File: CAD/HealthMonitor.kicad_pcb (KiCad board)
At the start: 2 copper layers, 20 x 30 mm, 28 parts, among them J1 USB_C_Receptacle_USB2.0, U1 ADP5092ACPZ-1-R7, U2 LTC4079IDD-PBF

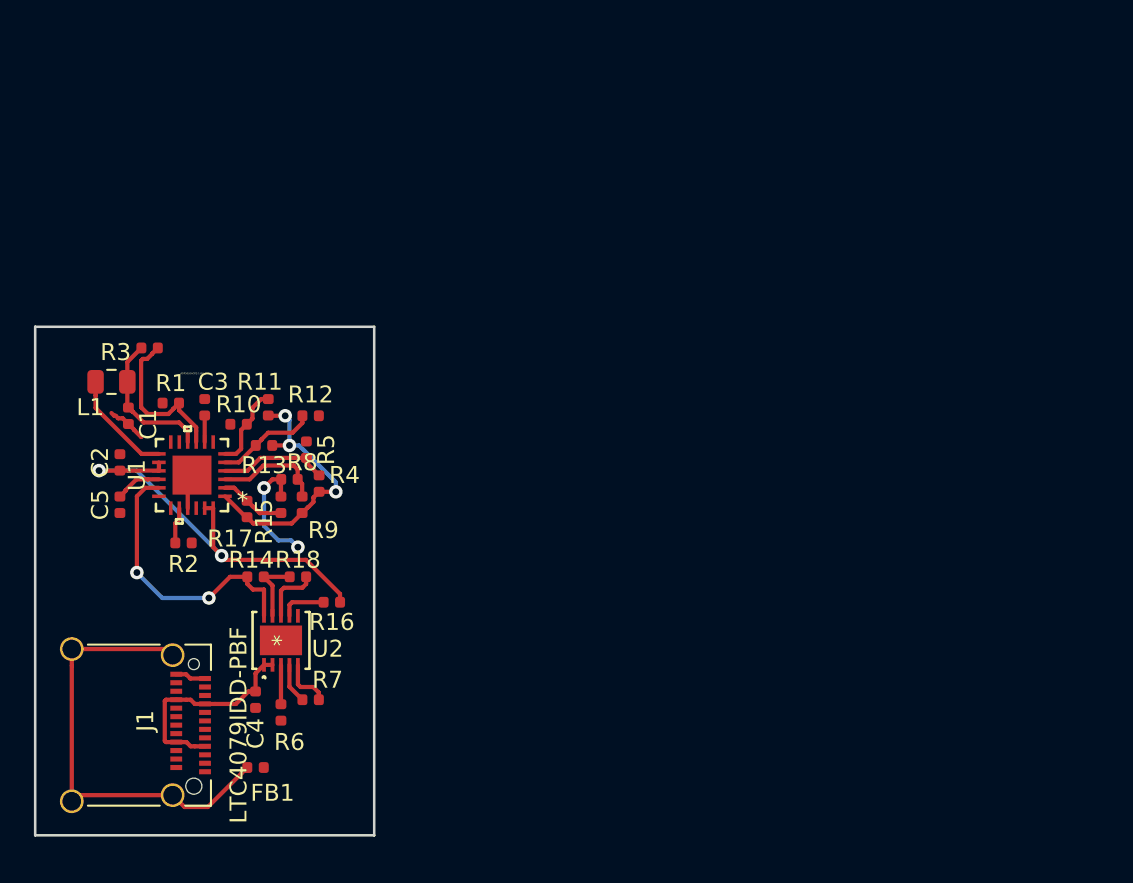
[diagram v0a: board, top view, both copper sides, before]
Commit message: Finished PCB Draft -- waiting for review
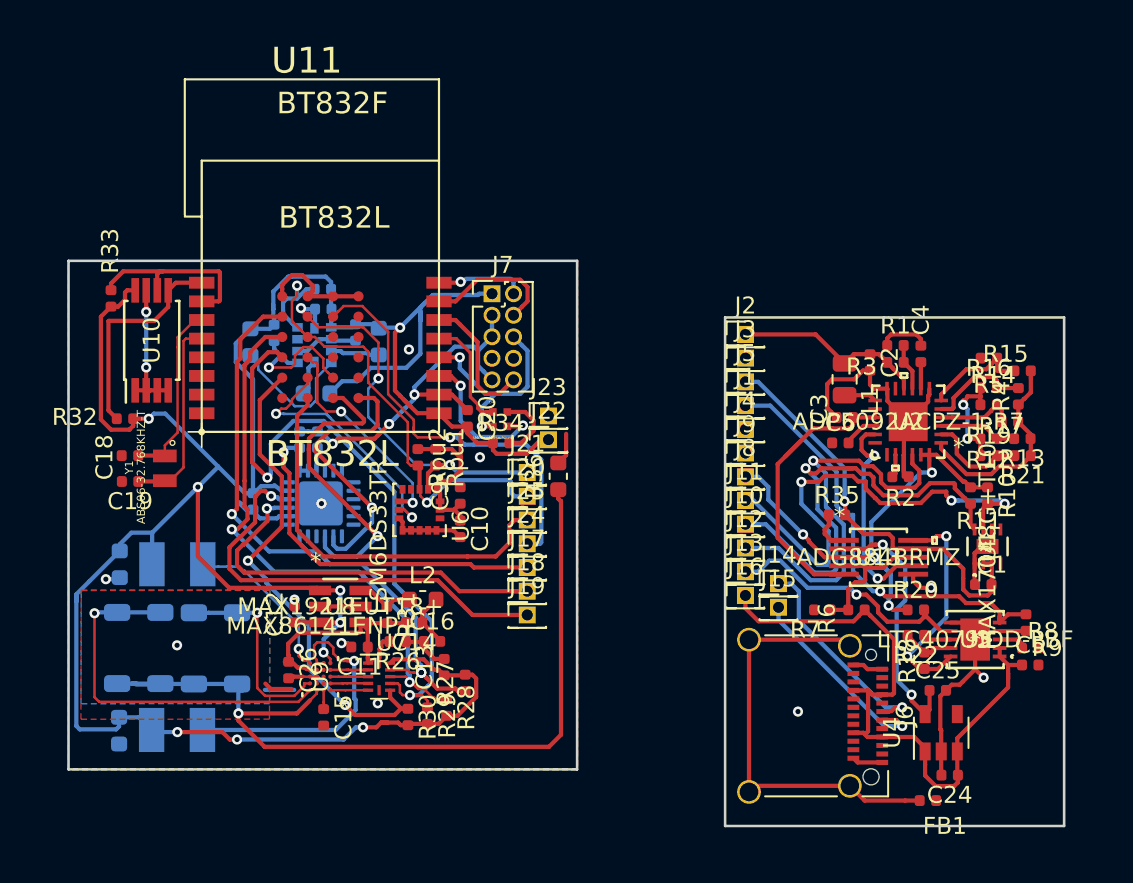
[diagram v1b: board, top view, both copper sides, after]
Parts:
- added C10: 10µF, Capacitor_SMD:C_0402_1005Metric, F.Cu at (125.1, 111.9)
- added C11: 0.1µF, Capacitor_SMD:C_0402_1005Metric, F.Cu at (119.1, 118.9)
- added C12: 4.7µF, Capacitor_SMD:C_0402_1005Metric, F.Cu at (115.3, 117.0)
- added C13: 0.1µF, Capacitor_SMD:C_0402_1005Metric, F.Cu at (124.1, 120.1)
- added C14: 5600pF, Capacitor_SMD:C_0402_1005Metric, F.Cu at (122.3, 117.5)
- added C15: 10µF 10V, Capacitor_SMD:C_0402_1005Metric, F.Cu at (117.0, 123.0)
- added C16: 4.7µF, Capacitor_SMD:C_0402_1005Metric, F.Cu at (123.4, 118.6)
- added C17: 22u, Capacitor_SMD:C_0603_1608Metric, B.Cu at (105.0, 123.8)
- added C18: 12p, Capacitor_SMD:C_0402_1005Metric, F.Cu at (105.6, 107.6)
- added C19: 12p, Capacitor_SMD:C_0402_1005Metric, F.Cu at (105.6, 109.1)
- added C20: 1u, Capacitor_SMD:C_0402_1005Metric, F.Cu at (125.5, 105.4)
- added C21: 1u, Capacitor_SMD:C_0402_1005Metric, B.Cu at (115.6, 106.7)
- added C22: 0.1u, Capacitor_SMD:C_0402_1005Metric, B.Cu at (116.7, 106.7)
- added C23: 1u, Capacitor_SMD:C_0402_1005Metric, B.Cu at (112.8, 110.3)
- added C24: 1u, Capacitor_SMD:C_0402_1005Metric, F.Cu at (153.9, 126.5)
- added C25: 1u, Capacitor_SMD:C_0402_1005Metric, F.Cu at (153.2, 121.5)
- added C26: 1µf 10V, Capacitor_SMD:C_0402_1005Metric, F.Cu at (115.0, 120.2)
- added C27: 22u, Capacitor_SMD:C_0603_1608Metric, B.Cu at (105.0, 114.0)
- added C6: 4.7u, Capacitor_SMD:C_0402_1005Metric, F.Cu at (147.5, 106.8)
- added C7: 1u, Capacitor_SMD:C_0402_1005Metric, B.Cu at (118.9, 100.3)
- added C9: 100nF, Capacitor_SMD:C_0402_1005Metric, F.Cu at (125.1, 110.0)
- added D1: LED_ir, Diode_SMD:D_0603_1608Metric, B.Cu at (116.6, 103.9)
- added D2: LED_green, Diode_SMD:D_0603_1608Metric, B.Cu at (112.7, 100.9)
- added D3: LED_green, Diode_SMD:D_0603_1608Metric, B.Cu at (120.3, 100.9)
- added D4: SML-LX0404SIUPGUSB, SML-LX0404SIUPGUSB:DIOC0404X01-4N, F.Cu at (127.4, 105.5)
- added D5: LED-LT PWSG-AABB-36-46-F, LED_SMD:LED_PLCC-2, B.Cu at (108.4, 114.0)
- added D6: VEMD5010X01, footprints:VEMD5010X01, B.Cu at (106.1, 119.0)
- added D7: LED_LY_P47F-TM, LED_SMD:LED_PLCC-2, B.Cu at (108.4, 123.8)
- added D8: VEMD5010X01, footprints:VEMD5010X01, B.Cu at (110.6, 119.0)
- added J10: SDA, Connector_PinHeader_1.27mm:PinHeader_1x01_P1.27mm_Vertical, F.Cu at (141.9, 111.7)
- added J11: SCL, Connector_PinHeader_1.27mm:PinHeader_1x01_P1.27mm_Vertical, F.Cu at (141.9, 110.2)
- added J12: DIS_SW, Connector_PinHeader_1.27mm:PinHeader_1x01_P1.27mm_Vertical, F.Cu at (141.9, 113.0)
- added J13: BAT_CHRG, Connector_PinHeader_1.27mm:PinHeader_1x01_P1.27mm_Vertical, F.Cu at (141.9, 114.5)
- added J14: USBDP, Connector_PinHeader_1.27mm:PinHeader_1x01_P1.27mm_Vertical, F.Cu at (143.8, 115.2)
- added J15: USBDM, Connector_PinHeader_1.27mm:PinHeader_1x01_P1.27mm_Vertical, F.Cu at (143.8, 116.5)
- added J16: USB_V, Connector_PinHeader_1.27mm:PinHeader_1x01_P1.27mm_Vertical, F.Cu at (141.9, 115.8)
- added J17: VBUS, Connector_PinHeader_1.27mm:PinHeader_1x01_P1.27mm_Vertical, F.Cu at (129.0, 114.2)
- added J18: D+, Connector_PinHeader_1.27mm:PinHeader_1x01_P1.27mm_Vertical, F.Cu at (129.0, 115.6)
- added J19: D-, Connector_PinHeader_1.27mm:PinHeader_1x01_P1.27mm_Vertical, F.Cu at (129.0, 117.0)
- added J2: TEG+, Connector_PinHeader_1.27mm:PinHeader_1x01_P1.27mm_Vertical, F.Cu at (141.9, 100.5)
- added J20: SDA, Connector_PinHeader_1.27mm:PinHeader_1x01_P1.27mm_Vertical, F.Cu at (129.0, 110.0)
- added J21: SCL, Connector_PinHeader_1.27mm:PinHeader_1x01_P1.27mm_Vertical, F.Cu at (129.0, 108.6)
- added J22: VCC, Connector_PinHeader_1.27mm:PinHeader_1x01_P1.27mm_Vertical, F.Cu at (130.3, 106.7)
- added J23: GND, Connector_PinHeader_1.27mm:PinHeader_1x01_P1.27mm_Vertical, F.Cu at (130.3, 105.3)
- added J24: BAT_CHRG, Connector_PinHeader_1.27mm:PinHeader_1x01_P1.27mm_Vertical, F.Cu at (129.0, 112.8)
- added J25: DIS_SW, Connector_PinHeader_1.27mm:PinHeader_1x01_P1.27mm_Vertical, F.Cu at (129.0, 111.4)
- added J3: TEG-, Connector_PinHeader_1.27mm:PinHeader_1x01_P1.27mm_Vertical, F.Cu at (141.9, 101.8)
- added J4: BAT-, Connector_PinHeader_1.27mm:PinHeader_1x01_P1.27mm_Vertical, F.Cu at (141.9, 106.0)
- added J5: BAT+, Connector_PinHeader_1.27mm:PinHeader_1x01_P1.27mm_Vertical, F.Cu at (141.9, 103.2)
- added J6: USB_C_Receptacle_USB2.0, Connector_USB:USB_C_Receptacle_Amphenol_12401610E4-2A_CircularHoles, F.Cu at (144.9, 123.0)
- added J7: Conn_02x05_Odd_Even, Connector_PinHeader_1.27mm:PinHeader_2x05_P1.27mm_Vertical, F.Cu at (127.0, 98.0)
- added J8: VCC, Connector_PinHeader_1.27mm:PinHeader_1x01_P1.27mm_Vertical, F.Cu at (141.9, 108.8)
- added J9: GND, Connector_PinHeader_1.27mm:PinHeader_1x01_P1.27mm_Vertical, F.Cu at (141.9, 107.5)
- added L2: 4.7µH, Inductor_SMD:L_0603_1608Metric, F.Cu at (122.9, 116.1)
- added R19: 3.32M, Resistor_SMD:R_0402_1005Metric, F.Cu at (156.2, 107.6)
- added R20: 2.4k, Resistor_SMD:R_0402_1005Metric, F.Cu at (151.9, 116.7)
- added R21: 6.65M, Resistor_SMD:R_0402_1005Metric, F.Cu at (158.2, 107.6)
- added R22: 412k, Resistor_SMD:R_0402_1005Metric, F.Cu at (151.9, 118.2)
- added R23: 10k, Resistor_SMD:R_0402_1005Metric, B.Cu at (117.0, 99.0)
- added R24: 10k, Resistor_SMD:R_0402_1005Metric, B.Cu at (117.0, 97.8)
- added R25: 10k, Resistor_SMD:R_0402_1005Metric, B.Cu at (114.1, 100.4)
- added R26: 50k, Resistor_SMD:R_0402_1005Metric, F.Cu at (121.4, 118.6)
- added R27: 50k, Resistor_SMD:R_0402_1005Metric, F.Cu at (125.4, 121.0)
- added R28: 50k, Resistor_SMD:R_0402_1005Metric, F.Cu at (124.3, 122.5)
- added R29: 50k, Resistor_SMD:R_0402_1005Metric, F.Cu at (123.1, 122.9)
- added R30: 50k, Resistor_SMD:R_0402_1005Metric, F.Cu at (122.0, 123.0)
- added R31: 4.75k, Resistor_SMD:R_0402_1005Metric, F.Cu at (120.8, 117.0)
- added R32: 10k, Resistor_SMD:R_0402_1005Metric, F.Cu at (105.3, 105.4)
- added R33: 10k, Resistor_SMD:R_0402_1005Metric, F.Cu at (104.5, 98.3)
- added R34: 6.6k, Resistor_SMD:R_0402_1005Metric, F.Cu at (127.5, 106.8)
- added R35: 10k, Resistor_SMD:R_0402_1005Metric, F.Cu at (147.3, 111.1)
- added R36: 0, Resistor_SMD:R_0603_1608Metric, F.Cu at (130.9, 108.8)
- added Rpu1: 10kOhms, Resistor_SMD:R_0402_1005Metric, F.Cu at (123.6, 107.7)
- added Rpu2: 10kOhms, Resistor_SMD:R_0402_1005Metric, F.Cu at (122.6, 107.7)
- added U10: AT24CS02-XHM, Package_SO:TSSOP-8_4.4x3mm_P0.65mm, F.Cu at (106.9, 100.8)
- added U11: BT832L, footprints:BT832-BT832L, F.Cu at (109.8, 106.2)
- added U12: CP2102N-A01-GQFN24, Package_DFN_QFN:QFN-24-1EP_4x4mm_P0.5mm_EP2.6x2.6mm, B.Cu at (116.8, 110.4)
- added U13: ADG884BRMZ, footprints:ADG884BRMZ, F.Cu at (149.8, 113.6)
- added U3: LTC4079IDD-PBF, footprints:LTC4079IDD-PBF, F.Cu at (155.4, 118.5)
- added U4: LD39015M33R, Package_TO_SOT_SMD:SOT-23-5, F.Cu at (153.4, 124.0)
- added U5: BH1792GLC, BH1790GLC-E2:PQFN70P280X280X100-10N, B.Cu at (116.5, 101.1)
- added U6: LSM6DS33TR, LSM6DS33TR:PQFN50P300X300X86-16N, F.Cu at (122.7, 110.8)
- added U7: TXB0104RUT, Package_DFN_QFN:Texas_R_PUQFN-N12, F.Cu at (120.3, 120.6)
- added U8: MAX1921EUT18+, footprints:MAX1921EUT18&plus_T, F.Cu at (118.0, 116.5)
- added U9: MAX86141ENP+, footprints:MAX86141ENP, F.Cu at (116.8, 120.6)
- added Y1: ABS06-32.768KHZ-T, ABS06-32.768KHZ-T:XTAL_ABS06-32.768KHZ-T, F.Cu at (107.7, 108.3)
- C1: value 10u -> 0.1u
- C3: value 10n -> 10u
- C4: value 1u -> 10n
- C5: value 4.7u -> 1u
- J1: value USB_C_Receptacle_USB2.0 -> BAT_T; footprint Connector_USB:USB_C_Receptacle_Amphenol_12401610E4-2A_CircularHoles -> Connector_PinHeader_1.27mm:PinHeader_1x01_P1.27mm_Vertical
- R10: value 3.01M -> 10k
- R11: value 6.98M -> 10k
- R12: value 3.32M -> 5M
- R13: value 6.65M -> 5M
- R14: value 1.07M -> 3.01M
- R15: value 3.57M -> 6.98M
- R16: value 2.4k -> 3.32M
- R17: value 6.49M -> 6.65M
- R18: value 412k -> 1.07M
- R6: value 3.3k -> 1M
- R7: value 10k -> 2M
- R8: value 5M -> 3.3k
- R9: value 5M -> 10k
- U1: value ADP5092ACPZ-1-R7 -> MAX17048G+T10; footprint footprints:ADP5092ACPZ-1-R7 -> footprints:MAX17048G+
- U2: value LTC4079IDD-PBF -> ADP5092ACPZ-1-R7; footprint footprints:LTC4079IDD-PBF -> footprints:ADP5092ACPZ-1-R7
- moved C5 54.5 mm to (158.7, 120.0), turned to 0 degrees
- moved C1 51.4 mm to (155.9, 115.2), turned to 0 degrees
- moved U1 47.1 mm to (156.2, 113.0), turned to 90 degrees
- moved R17 46.0 mm to (158.0, 104.1)
- moved R14 45.1 mm to (156.3, 101.8), turned to 0 degrees
- moved R8 44.8 mm to (158.7, 119.0)
- moved R13 44.7 mm to (158.2, 106.6)
- moved C2 44.6 mm to (149.2, 102.1), turned to 270 degrees
- moved R15 44.5 mm to (158.2, 102.6), turned to 180 degrees
- moved R10 44.4 mm to (156.2, 110.0), turned to 270 degrees
- moved C4 44.2 mm to (152.2, 101.6), turned to 90 degrees
- moved R3 44.0 mm to (150.8, 102.1)
- moved R9 43.3 mm to (158.4, 117.5)
- moved L1 43.3 mm to (147.8, 103.1), turned to 90 degrees
- moved R1 42.9 mm to (150.8, 101.1)
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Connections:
- C1 pad 1: /power/TEG+ -> GND
- C1 pad 2: GND -> /power/BAT+
- C2 pad 1: +3V3 -> /power/TEG+
- C3 pad 1: Net-(C3-Pad1) -> /power/EH_3v3
- C5 pad 1: GND -> /power/USB_VBUS
- C5 pad 2: Net-(C5-Pad2) -> GND
- R10 pad 1: GND -> +3V3
- R10 pad 2: Net-(R10-Pad2) -> /SCL
- R11 pad 1: /power/REF -> +3V3
- R11 pad 2: Net-(R10-Pad2) -> /SDA
- R14 pad 1: Net-(R14-Pad1) -> GND
- R14 pad 2: /power/BAT+ -> Net-(R14-Pad2)
- R15 pad 1: GND -> /power/REF
- R15 pad 2: Net-(R15-Pad2) -> Net-(R14-Pad2)
- R16 pad 1: +3V3 -> GND
- R16 pad 2: /power/BAT_CHRG -> Net-(R16-Pad2)
- R17 pad 2: Net-(R15-Pad2) -> Net-(R16-Pad2)
- R18 pad 2: Net-(R14-Pad1) -> /power/BAT_USB
- R6 pad 1: Net-(R6-Pad1) -> /power/USB_VBUS
- R6 pad 2: GND -> /power/B_CONN
- R7 pad 1: Net-(R7-Pad1) -> /power/B_CONN
- R7 pad 2: /power/BAT_T -> GND
- R8 pad 1: GND -> Net-(R8-Pad1)
- R8 pad 2: Net-(R8-Pad2) -> GND
- R9 pad 1: /power/REF -> Net-(R9-Pad1)
- R9 pad 2: Net-(R8-Pad2) -> /power/BAT_T
- U1 pad 1: /power/REF -> GND
- U1 pad 2: Net-(R15-Pad2) -> /power/BAT+
- U1 pad 3: Net-(R8-Pad2) -> /power/BAT+
- U1 pad 4: Net-(R4-Pad1) -> GND
- U1 pad 5: Net-(R12-Pad2) -> Net-(U1-Pad5)
- U1 pad 6: Net-(R10-Pad2) -> GND
- U1 pad 7: GND -> /SCL
- U1 pad 8: Net-(C3-Pad1) -> /SDA
- U1 pad 9: Net-(R1-Pad2) -> GND
- U2 pad 1: Net-(C4-Pad1) -> /power/REF
- U2 pad 10: /power/BAT+ -> /power/TEG+
- U2 pad 11: GND -> /power/REG_GOOD
- U2 pad 2: Net-(C4-Pad1) -> Net-(R19-Pad2)
- U2 pad 3: Net-(R6-Pad1) -> Net-(R12-Pad2)
- U2 pad 4: Net-(R7-Pad1) -> Net-(R4-Pad1)
- U2 pad 5: /power/BAT_T -> Net-(R16-Pad2)
- U2 pad 6: GND -> Net-(R14-Pad2)
- U2 pad 7: /power/BAT_CHRG -> GND
- U2 pad 8: Net-(R18-Pad1) -> Net-(C4-Pad1)
- U2 pad 9: Net-(R14-Pad1) -> Net-(R1-Pad2)
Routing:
- net +3V3: track 25.3 -> 196.8 mm, vias 2 -> 13
- net GND: track 13.2 -> 111.9 mm, vias 2 -> 17
- net /power/USB_VBUS: track 0.00 -> 62.8 mm, vias 0 -> 1
- net /SDA: track 0.00 -> 59.2 mm, vias 0 -> 3
- net Net-(D6-Pad3): track 0.00 -> 55.2 mm, vias 0 -> 2
- net /SCL: track 0.00 -> 54.5 mm, vias 0 -> 6
- net /DIS_SW: track 0.00 -> 47.3 mm, vias 0 -> 1
- net /BAT_CHRG: track 0.00 -> 40.4 mm, vias 0 -> 2
- net /SoC/SDI: track 0.00 -> 38.3 mm, vias 0 -> 2
- net /programmer/D-: track 0.00 -> 37.8 mm, vias 0 -> 2
- net /programmer/D+: track 0.00 -> 36.5 mm, vias 0 -> 2
- net /SoC/SCLK: track 0.00 -> 35.6 mm, vias 0 -> 3
- net /SoC/SDO: track 0.00 -> 34.1 mm, vias 0 -> 2
- net /SoC/CSB: track 0.00 -> 29.0 mm, vias 0 -> 2
- net /power/BAT_T: track 3.01 -> 25.9 mm, vias 0 -> 1
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- added copper zone on B.Cu, net Net-(D6-Pad3)
- added copper zone on F.Cu, net Net-(D6-Pad3)
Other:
- board size 20 x 30 mm -> 58.7 x 33.3 mm
- net class Default: via_dia 0.8 -> 0.6; via_drill 0.4 -> 0.3
- rule trace_min: 0.2 -> 0.1
